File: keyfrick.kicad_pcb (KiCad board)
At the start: 2 copper layers, 96 x 34 mm, 13 parts, among them SW1 SW_Push, SW2 SW_Push, SW3 SW_Push, SW4 SW_Push, U1 XIAO-RP2040-DIP

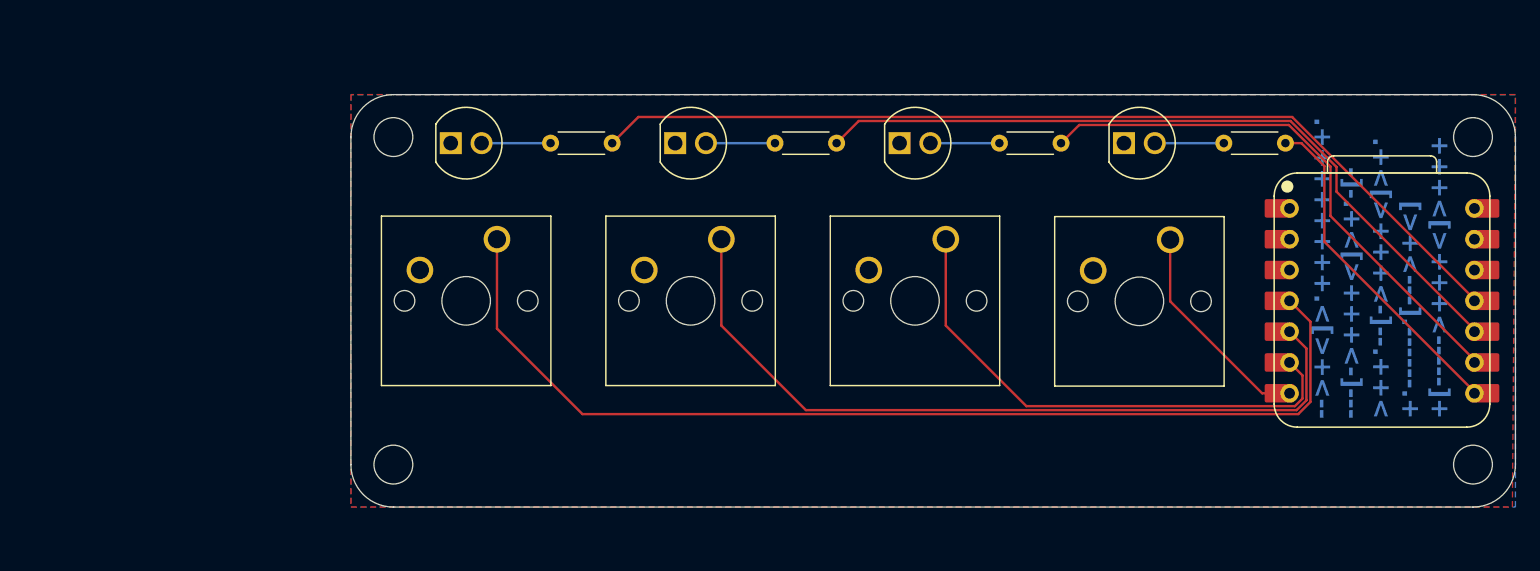
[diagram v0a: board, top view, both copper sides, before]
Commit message: Add files via upload
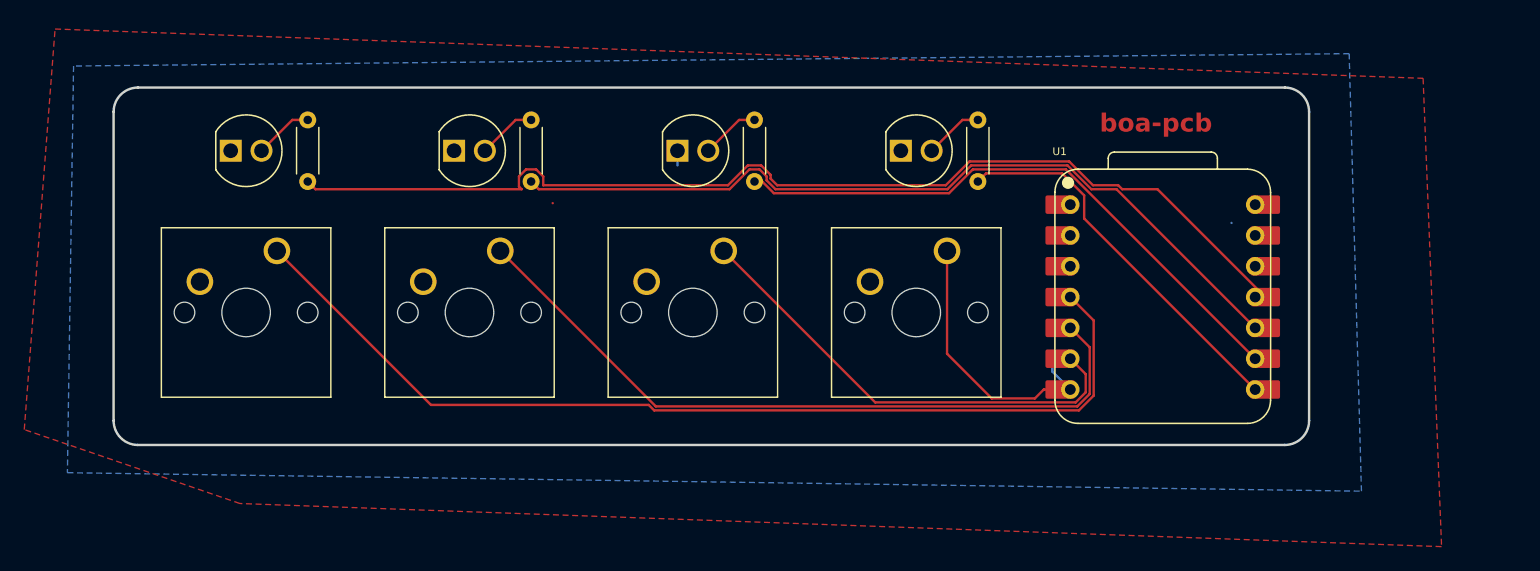
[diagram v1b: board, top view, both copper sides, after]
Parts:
- moved R4 20.4 mm to (146.7, 45.1), turned to -90 degrees
- moved R3 20.3 mm to (128.3, 45.1), turned to -90 degrees
- moved R2 20.2 mm to (109.9, 45.1), turned to -90 degrees
- moved R1 20.1 mm to (91.4, 45.1), turned to -90 degrees
- moved SW4 18.4 mm to (144.1, 55.9)
- moved D4 18.4 mm to (141.6, 47.6)
- moved SW3 18.3 mm to (125.7, 55.9)
- moved D3 18.3 mm to (123.2, 47.6)
- moved SW2 18.3 mm to (107.3, 55.9)
- moved D2 18.2 mm to (104.8, 47.6)
- moved SW1 18.2 mm to (88.9, 55.9)
- moved D1 18.2 mm to (86.4, 47.6)
- moved U1 18.1 mm to (161.9, 59.7)
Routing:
- net d1: track 78.3 -> 89.6 mm
- net sw4: track 17.2 -> 24.9 mm
- net d2: track 62.6 -> 68.7 mm
- net d4: track 28.4 -> 32.5 mm
- net sw1: track 86.8 -> 83.0 mm
- net d3: track 46.0 -> 49.8 mm
- net sw2: track 64.8 -> 61.3 mm
- net sw3: track 43.0 -> 39.5 mm
- net GND: track 0.06 -> 2.30 mm
- net unconnected-(U1-VBUS-Pad14): track 0.00 -> 0.84 mm
- net unconnected-(U1-GPIO28/ADC2/A2-Pad3): track 0.00 -> 0.84 mm
- net unconnected-(U1-GPIO27/ADC1/A1-Pad2): track 0.00 -> 0.84 mm
- net unconnected-(U1-GPIO26/ADC0/A0-Pad1): track 0.00 -> 0.84 mm
- net unconnected-(U1-3V3-Pad12): track 0.00 -> 0.84 mm
- net Net-(D2-PadA): track 5.69 -> 4.86 mm
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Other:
- board size 96 x 34 mm -> 98.6 x 29.5 mm
- board text added: "boa-pcb"
- board text removed: "+[----->+++<]>+++ +.------.[--->+<] >++.--[->+++<]>+. ---[->+++<]>+.-[- -->+<]>.++++++++."
- board text removed: "keyf*ck"
- board text removed: "| x o o o | o o o x | o x o o | o o x o | x x o o | o o x x | x o x o | o x o x | x x x x | < | > | + | - | [ | ] | . | , | ⌫"
